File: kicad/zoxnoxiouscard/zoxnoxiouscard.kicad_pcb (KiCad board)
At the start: 4 copper layers, 80 x 80 mm, 21 parts, among them J1 Conn_01x01, J2 Conn_01x02, J3 Conn_02x20_Odd_Even, U13 LM4040AIM3-2.5, U14 AD5328, U15 M24C02-WMN, U7 PCA9555D

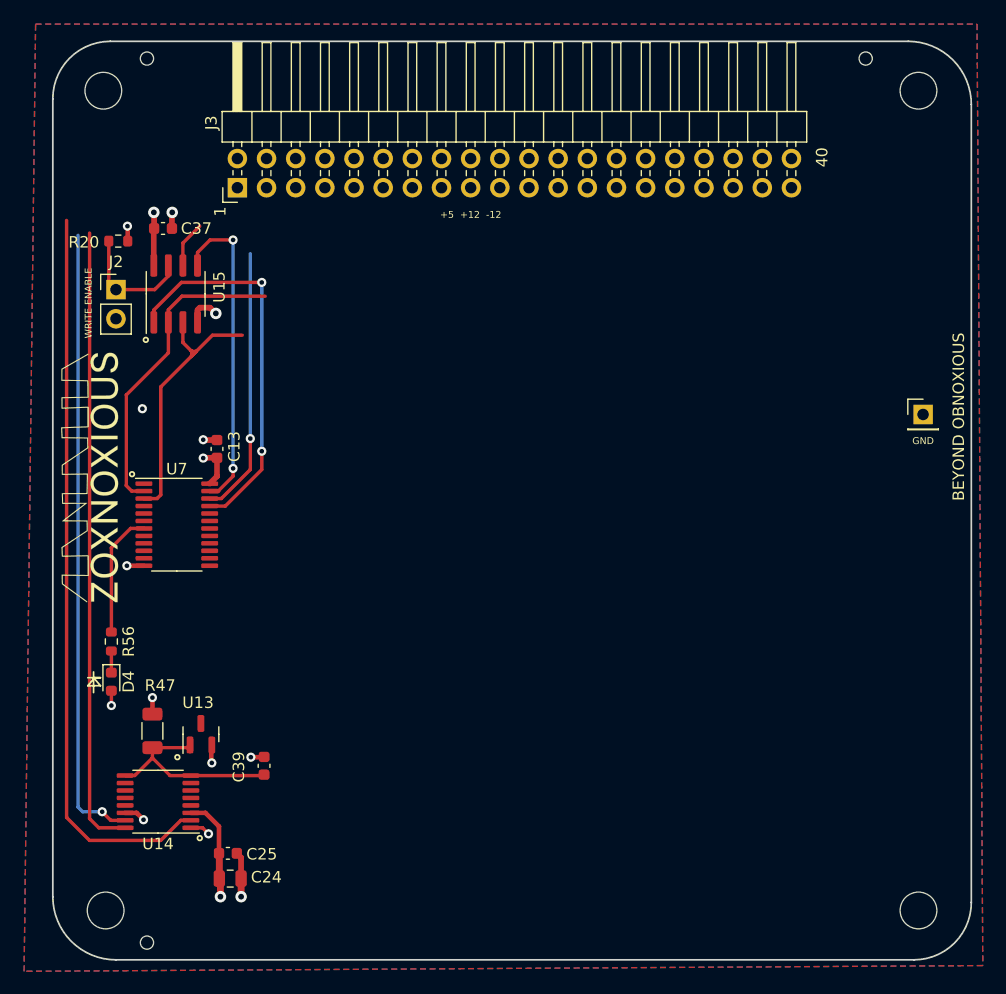
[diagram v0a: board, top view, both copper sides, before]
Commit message: modified template
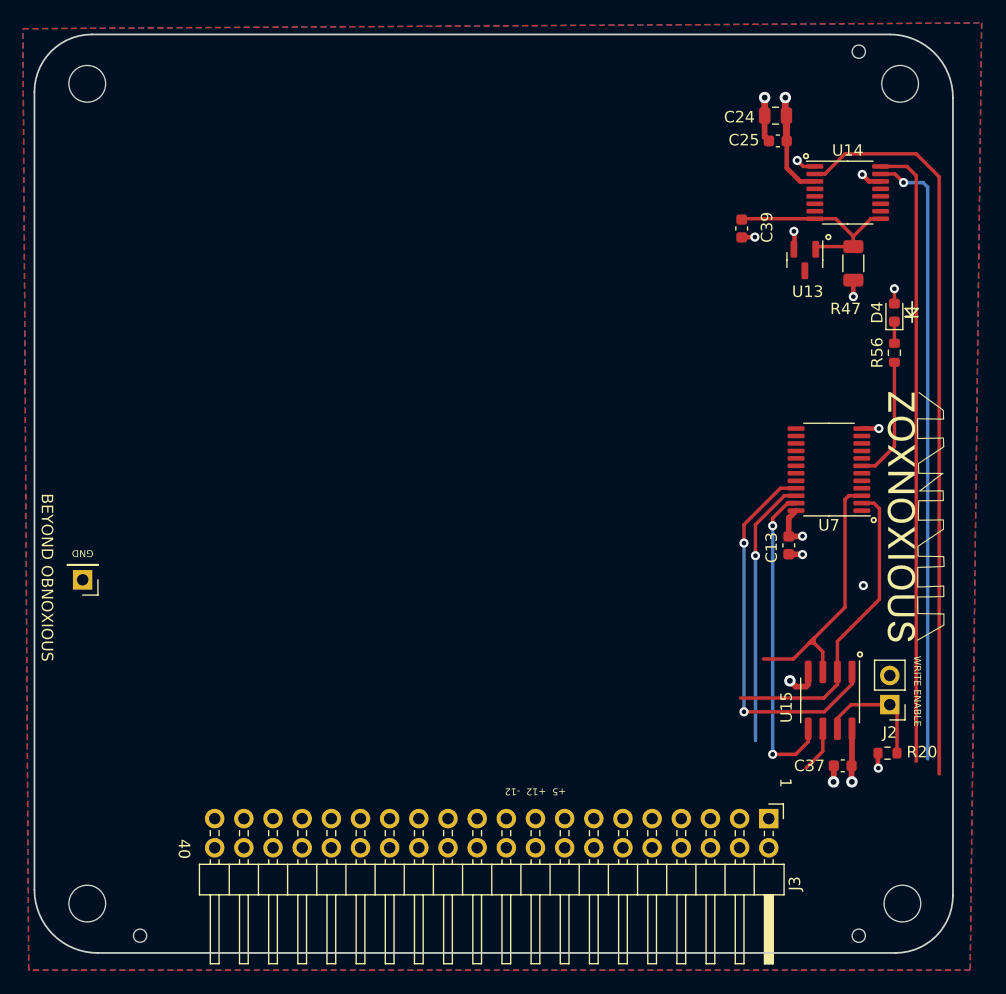
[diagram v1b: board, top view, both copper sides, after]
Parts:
- moved H4 102.1 mm to (70.0, 29.2), turned to 180 degrees
- moved H3 101.3 mm to (70.0, 100.6), turned to 180 degrees
- moved H2 99.9 mm to (140.8, 29.2), turned to 180 degrees
- moved H1 99.3 mm to (141.0, 100.6), turned to 180 degrees
- moved C24 81.7 mm to (129.9, 32.0), turned to 180 degrees
- moved R20 80.5 mm to (139.7, 87.5), turned to 0 degrees
- moved U14 80.1 mm to (136.2, 38.7), turned to 0 degrees
- moved C25 78.4 mm to (130.2, 34.2), turned to 180 degrees
- moved J2 76.5 mm to (139.9, 83.3), turned to 180 degrees
- moved C37 75.5 mm to (135.8, 88.6), turned to 0 degrees
- moved D4 75.4 mm to (140.3, 49.1), turned to 90 degrees
- moved J1 74.6 mm to (69.6, 72.4), turned to 180 degrees
- moved R47 73.4 mm to (136.7, 44.8), turned to 90 degrees
- moved R56 72.7 mm to (140.3, 52.6), turned to -90 degrees
- moved G*** 72.1 mm to (142.2, 66.9), turned to -90 degrees
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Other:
- outline, holes or cut-outs redrawn
